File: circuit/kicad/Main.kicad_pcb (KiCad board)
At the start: 2 copper layers, 110.8 x 117 mm, 104 parts, among them J1 SH3, J10 PA3, J11 SH4, J2 SH3, J3 FFC6, J4 SH6, J5 FTSH2x5, J6 FFC4, J7 SH4, J8 FFC12, J9 FTSH2x5, Q1 TEMT7100X01, Q10 2N7002T, Q11 TEMT7100X01, Q12 TEMT7100X01, Q13 TEMT7100X01, Q2 TEMT7100X01, Q3 TEMT7100X01, Q4 TEMT7100X01, Q5 TEMT7100X01, Q6 TEMT7100X01, Q7 TEMT7100X01, Q8 TEMT7100X01, Q9 TEMT7100X01, SW1 SKRPABE010, U1 ASTMLPA-16MHz-LJ-E-T, U2 STM32F405RGTx, U3 ICM-20648

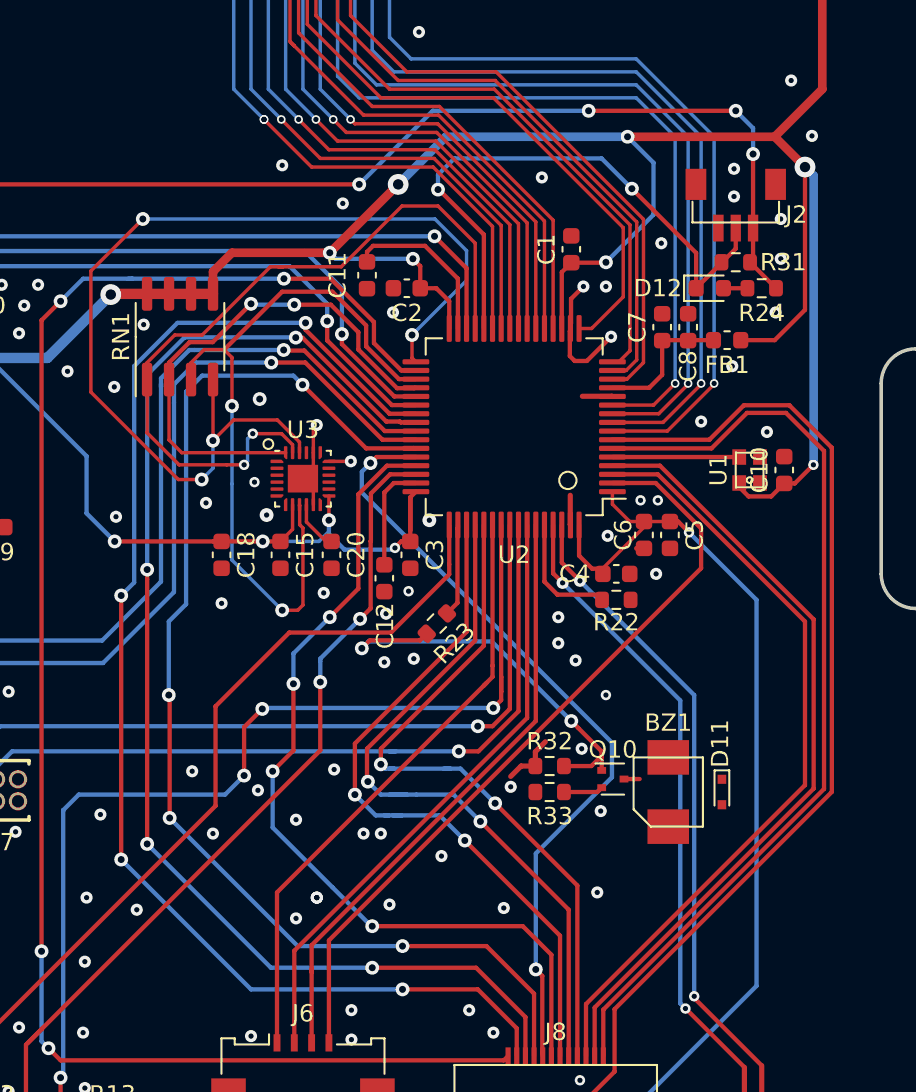
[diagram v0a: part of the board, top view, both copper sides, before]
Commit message: 後はガーバデータ出してロゴ刺すだけ
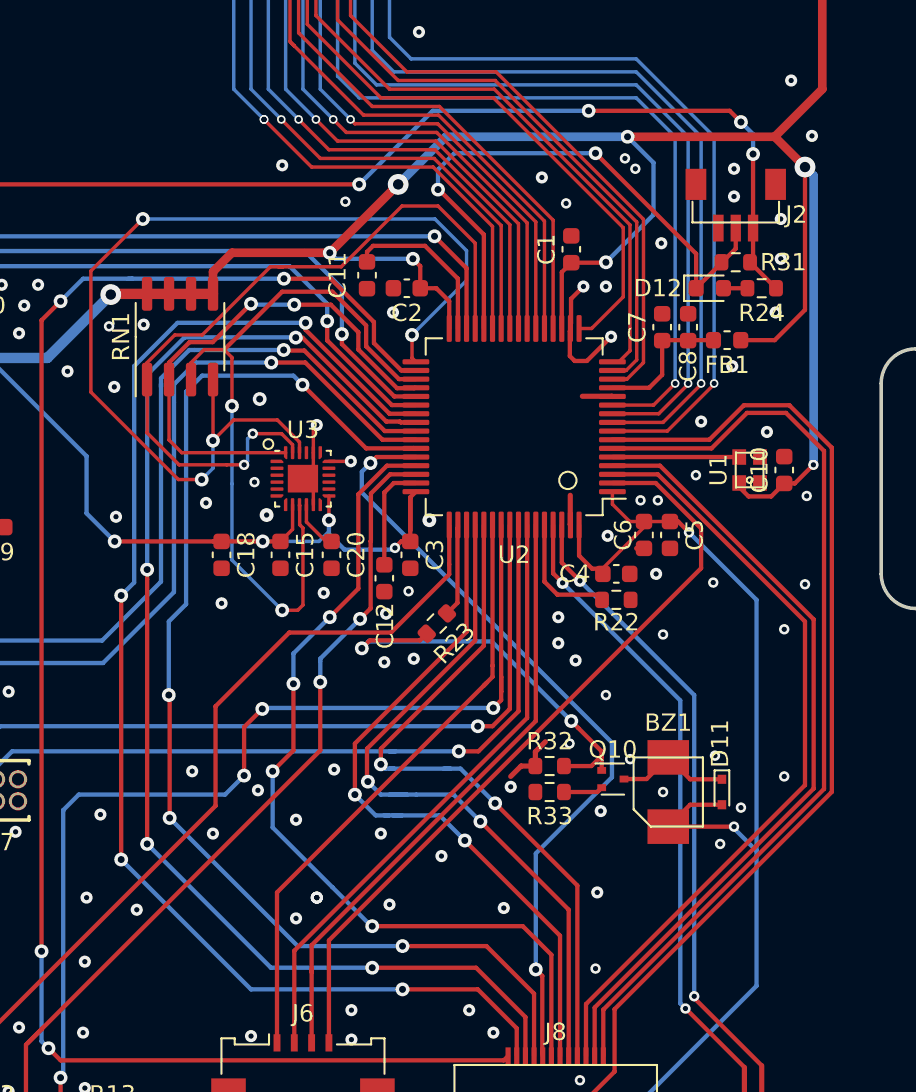
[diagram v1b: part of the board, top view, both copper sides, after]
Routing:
- net +3V3: track 442.9 -> 452.3 mm, vias 18 -> 19
- net Net-(BZ1-Pad2): track 0.90 -> 6.70 mm
- net GND: vias 147 -> 163
